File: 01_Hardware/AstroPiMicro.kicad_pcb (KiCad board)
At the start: 2 copper layers, 65 x 50.2 mm, 53 parts, among them J1 RPi Connector, J10 6-pin JST PH, J2 USB_C_Receptacle_USB2.0, J3 2-pin JST PH, J4 4-pin JST SH, J5 4-pin JST SH, J6 11-pin JST PH, J7 3-pin JST PH, J8 3-pin JST PH, J9 6-pin JST PH, SW1 SW-ON-OFF, U1 LM809, U2 STM32G431KBTx, U3 MCP73831-2-OT, U4 TPS61090, U5 Joystick, Y1 16MHz

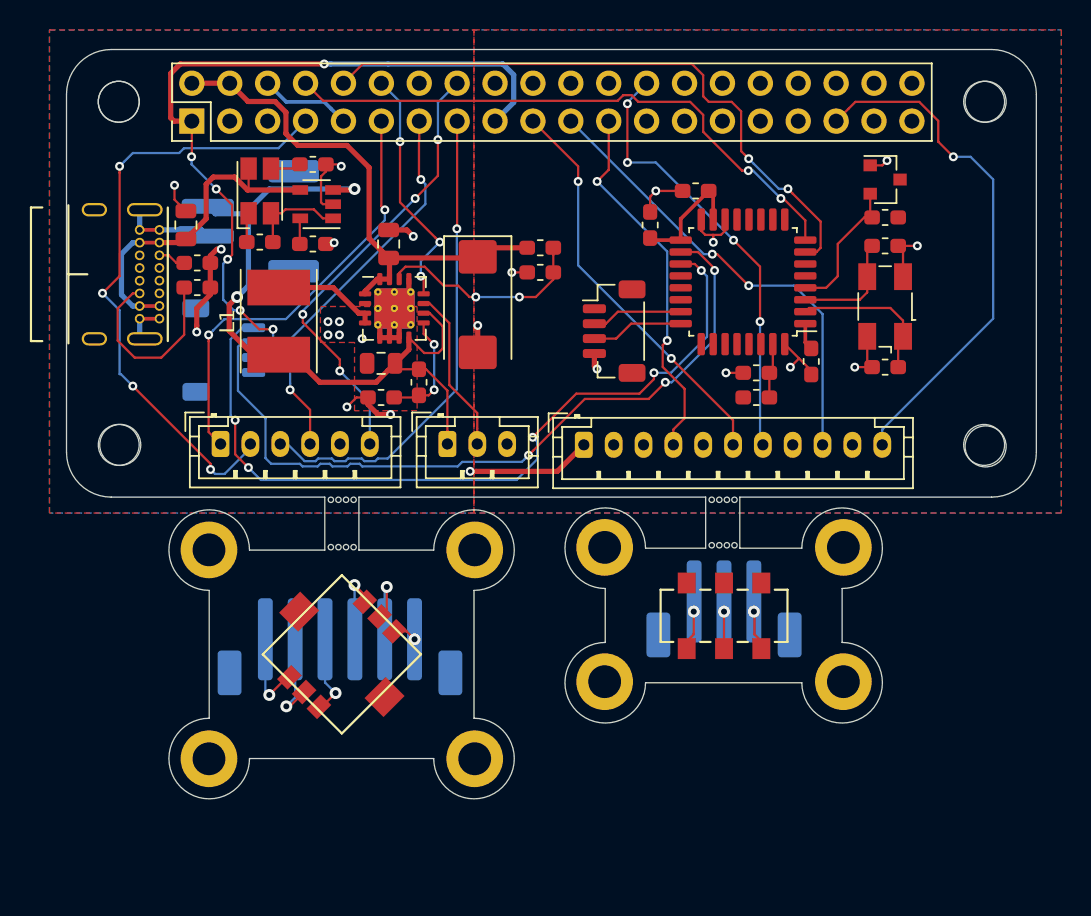
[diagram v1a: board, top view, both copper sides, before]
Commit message: Started on HW version 2
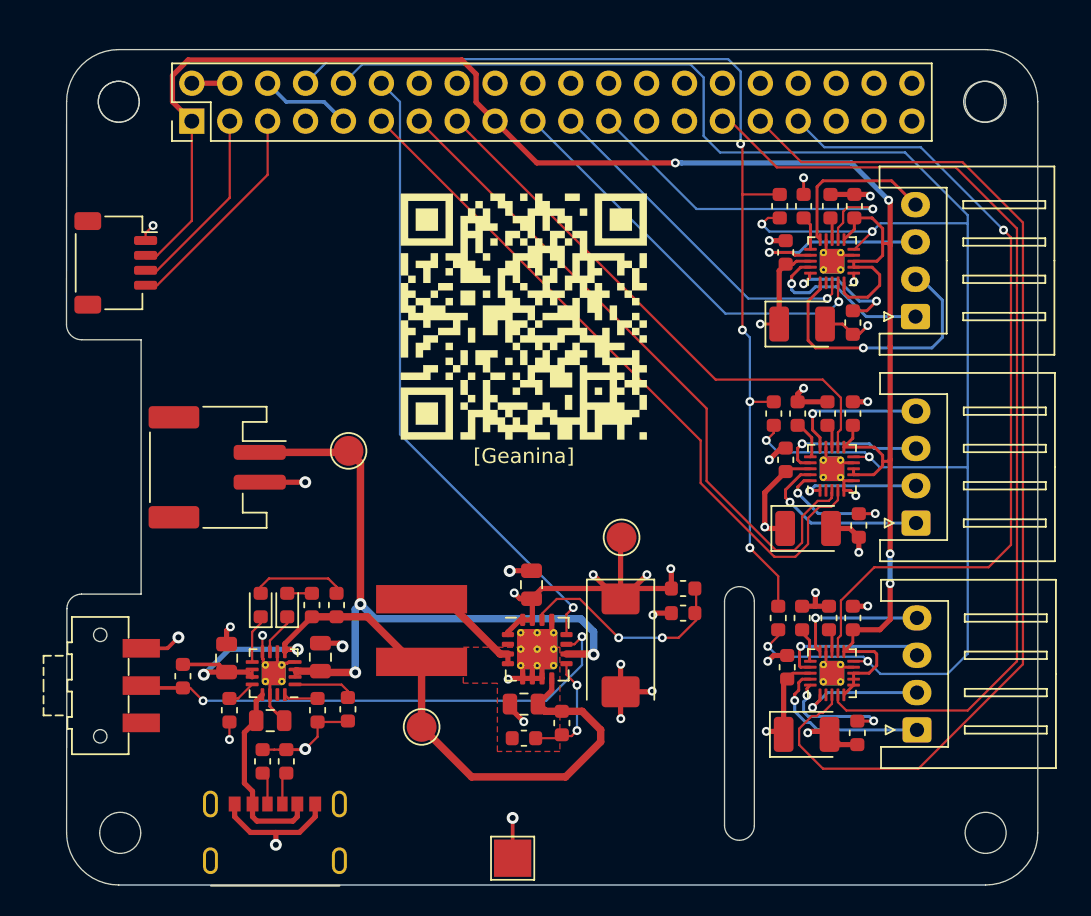
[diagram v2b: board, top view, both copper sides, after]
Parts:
- removed the ? at (53.6, 75.5)
- removed the ? at (111.6, 75.6)
- removed G***: LOGO, astropi:qr
- removed J10: 6-pin JST PH, Connector_JST:JST_PH_B6B-PH-K_1x06_P2.00mm_Vertical
- removed J8: 3-pin JST PH, Connector_JST:JST_PH_B3B-PH-SM4-TB_1x03-1MP_P2.00mm_Vertical
- removed J9: 6-pin JST PH, Connector_JST:JST_PH_B6B-PH-SM4-TB_1x06-1MP_P2.00mm_Vertical
- removed REF** (x8): MountingHole_2.2mm_M2_ISO14580_Pad, MountingHole:MountingHole_2.2mm_M2_ISO14580_Pad
- removed Y1: 16MHz, Crystal:Crystal_SMD_Abracon_ABM3B-4Pin_5.0x3.2mm
- added ?: , RPi_Hat:RPi_Hat_Mounting_Hole, F.Cu at (53.6, 101.5)
- added ?: , RPi_Hat:RPi_Hat_Mounting_Hole, F.Cu at (111.6, 101.5)
- added C11: 100nF, Capacitor_SMD:C_0603_1608Metric, F.Cu at (102.7, 73.4)
- added C12: 100nF, Capacitor_SMD:C_0603_1608Metric, F.Cu at (98.2, 62.6)
- added C13: 47uF, Capacitor_Tantalum_SMD:CP_EIA-3528-15_AVX-H, F.Cu at (99.3, 67.4)
- added C14: 100nF, Capacitor_SMD:C_0603_1608Metric, F.Cu at (101.2, 59.5)
- added C15: 100nF, Capacitor_SMD:C_0603_1608Metric, F.Cu at (102.7, 87.1)
- added C16: 100nF, Capacitor_SMD:C_0603_1608Metric, F.Cu at (98.3, 90.4)
- added C17: 47uF, Capacitor_Tantalum_SMD:CP_EIA-3528-15_AVX-H, F.Cu at (99.6, 94.9)
- added C18: 100nF, Capacitor_SMD:C_0603_1608Metric, F.Cu at (101.1, 87.1)
- added C3: 4.7uF, Capacitor_SMD:C_0805_2012Metric, F.Cu at (67.0, 89.7)
- added D2: Orange, LED_SMD:LED_0603_1608Metric, F.Cu at (63.0, 86.2)
- added QR*****: MiniCalinGeani, astropi:MiniCalinGeani, F.Cu at (80.7, 66.9)
- added R11: 0.75, Resistor_SMD:R_0603_1608Metric, F.Cu at (99.0, 73.4)
- added R14: 0.75, Resistor_SMD:R_0603_1608Metric, F.Cu at (103.1, 80.9)
- added R15: 1k, Resistor_SMD:R_0603_1608Metric, F.Cu at (97.8, 59.5)
- added R16: 220m, Resistor_SMD:R_0603_1608Metric, F.Cu at (99.4, 59.5)
- added R17: 220m, Resistor_SMD:R_0603_1608Metric, F.Cu at (102.7, 67.3)
- added R18: 1k, Resistor_SMD:R_0603_1608Metric, F.Cu at (97.7, 87.1)
- added R19: 220m, Resistor_SMD:R_0603_1608Metric, F.Cu at (99.3, 87.1)
- added R20: 220m, Resistor_SMD:R_0603_1608Metric, F.Cu at (103.0, 94.8)
- added R21: 10k, Resistor_SMD:R_0603_1608Metric, F.Cu at (57.8, 91.0)
- added TP1: TP_VBAT, TestPoint:TestPoint_Pad_D2.0mm, F.Cu at (68.9, 75.9)
- added TP2: TP_Supply, TestPoint:TestPoint_Pad_D2.0mm, F.Cu at (73.8, 94.4)
- added TP3: TP_5V, TestPoint:TestPoint_Pad_D2.0mm, F.Cu at (87.2, 81.7)
- added TP4: TP_GND, TestPoint:TestPoint_Pad_2.5x2.5mm, F.Cu at (79.9, 103.2)
- C1: value 27pF -> 100nF; footprint Capacitor_SMD:C_0603_1608Metric_Pad1.05x0.95mm_HandSolder -> Capacitor_SMD:C_0603_1608Metric
- C10: footprint Capacitor_Tantalum_SMD:CP_EIA-7343-31_Kemet-D_Pad2.25x2.55mm_HandSolder -> Capacitor_Tantalum_SMD:CP_EIA-7343-15_Kemet-W
- C2: value 27pF -> 1uF; footprint Capacitor_SMD:C_0603_1608Metric_Pad1.05x0.95mm_HandSolder -> Capacitor_SMD:C_0805_2012Metric
- C4: value 100nF -> 10uF; footprint Capacitor_SMD:C_0603_1608Metric_Pad1.05x0.95mm_HandSolder -> Capacitor_SMD:C_0805_2012Metric
- C5: value 10uF -> 100nF; footprint Capacitor_SMD:C_0805_2012Metric -> Capacitor_SMD:C_0603_1608Metric
- C6: value 100nF -> 47uF; footprint Capacitor_SMD:C_0603_1608Metric_Pad1.05x0.95mm_HandSolder -> Capacitor_Tantalum_SMD:CP_EIA-3528-15_AVX-H
- C7: footprint Capacitor_SMD:C_0603_1608Metric_Pad1.05x0.95mm_HandSolder -> Capacitor_SMD:C_0603_1608Metric
- D1: value Status LED -> Green; footprint LED_SMD:LED_Avago_PLCC4_3.2x2.8mm_CW -> LED_SMD:LED_0603_1608Metric
- J2: value USB_C_Receptacle_USB2.0 -> SHOU_HAN_TYPE-C_6P; footprint astropi:USB_C_GCT_USB4085 -> astropi:SHOU HAN TYPE-C 6P
- J3, J4: moved to F.Cu
- J5: value 4-pin JST SH -> Stepper_Focus; footprint Connector_JST:JST_SH_BM04B-SRSS-TB_1x04-1MP_P1.00mm_Vertical -> Connector_JST:JST_XH_S4B-XH-A_1x04_P2.50mm_Horizontal
- J6: value 11-pin JST PH -> Stepper_Azimuth; footprint Connector_JST:JST_PH_B11B-PH-K_1x11_P2.00mm_Vertical -> Connector_JST:JST_XH_S4B-XH-A_1x04_P2.50mm_Horizontal
- J7: value 3-pin JST PH -> Stepper_Altitude; footprint Connector_JST:JST_PH_B3B-PH-K_1x03_P2.00mm_Vertical -> Connector_JST:JST_XH_S4B-XH-A_1x04_P2.50mm_Horizontal
- L1: value 6.8uH -> 10uH; footprint Inductor_SMD:L_Taiyo-Yuden_NR-50xx_HandSoldering -> astropi:VLS6045EX-100M
- R1: value 10k -> 1.1k; footprint Resistor_SMD:R_0603_1608Metric_Pad1.05x0.95mm_HandSolder -> Resistor_SMD:R_0603_1608Metric
- R10, R12, R13, R4, R5, R7, R8, R9: footprint Resistor_SMD:R_0603_1608Metric_Pad1.05x0.95mm_HandSolder -> Resistor_SMD:R_0603_1608Metric
- R2: value 10k -> 1k; footprint Resistor_SMD:R_0603_1608Metric_Pad1.05x0.95mm_HandSolder -> Resistor_SMD:R_0603_1608Metric
- R3: value 10k -> 1.5k; footprint Resistor_SMD:R_0603_1608Metric_Pad1.05x0.95mm_HandSolder -> Resistor_SMD:R_0603_1608Metric
- R6: value 2k -> 10k; footprint Resistor_SMD:R_0603_1608Metric_Pad1.05x0.95mm_HandSolder -> Resistor_SMD:R_0603_1608Metric
- SW1: value SW-ON-OFF -> SW_SPDT; footprint astropi:SSSS213202 -> Button_Switch_SMD:SW_SPDT_CK-JS102011SAQN
- U1: value LM809 -> BQ24074RGT; footprint Package_TO_SOT_SMD:SOT-23 -> Package_DFN_QFN:VQFN-16-1EP_3x3mm_P0.5mm_EP1.6x1.6mm_ThermalVias
- U2: value STM32G431KBTx -> TMC2300; footprint Package_QFP:LQFP-32_7x7mm_P0.8mm -> Package_DFN_QFN:QFN-20-1EP_3x3mm_P0.4mm_EP1.65x1.65mm_ThermalVias
- U3: value MCP73831-2-OT -> TMC2300; footprint Package_TO_SOT_SMD:SOT-23-5 -> Package_DFN_QFN:QFN-20-1EP_3x3mm_P0.4mm_EP1.65x1.65mm_ThermalVias
- U5: value Joystick -> TMC2300; footprint astropi:SKRHAAE010 -> Package_DFN_QFN:QFN-20-1EP_3x3mm_P0.4mm_EP1.65x1.65mm_ThermalVias
- moved R1 55.0 mm to (60.9, 93.3), turned to 90 degrees
- moved U1 52.7 mm to (63.9, 90.8), turned to 180 degrees
- moved C2 52.1 mm to (63.6, 94.0)
- moved C4 43.9 mm to (60.7, 89.8), turned to 90 degrees
- moved C5 43.2 mm to (98.2, 76.5)
- moved SW1 39.4 mm to (52.3, 91.6), turned to 270 degrees
- moved J2 38.1 mm to (64.0, 99.6), turned to 0 degrees
- moved J7 36.8 mm to (107.0, 94.6), turned to 90 degrees
- moved R3 36.1 mm to (66.8, 93.3), turned to 90 degrees
- moved U3 34.8 mm to (101.3, 63.2), turned to 90 degrees
- moved R4 33.7 mm to (63.1, 96.7), turned to 270 degrees
- moved U5 32.9 mm to (101.3, 90.8), turned to 90 degrees
- moved R5 32.3 mm to (64.7, 96.7), turned to 270 degrees
- moved R6 31.3 mm to (68.9, 93.2), turned to 270 degrees
- moved R8 29.6 mm to (68.1, 86.2), turned to 90 degrees
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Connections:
- C1 pad 1: Net-(C1-Pad1) -> +3V3
- C2 pad 1: Net-(C2-Pad1) -> VBUS
- C4 pad 1: +3V3 -> /Vsupply
- C5 pad 1: VBUS -> +5V
- C6 pad 1: +3V3 -> +5V
- C7 pad 1: +3V3 -> Net-(C7-Pad1)
- C8 pad 1: +BATT -> /Vsupply
- D1 pad 2: VBUS -> Net-(D1-Pad2)
- J1 pad 10: /PI_UART_RX -> /UART_RX
- J1 pad 11: /GPIO17 -> /STEP_Focus
- J1 pad 13: /GPIO27 -> /DIR_Focus
- J1 pad 15: /GPIO22 -> /ERR_Focus
- J1 pad 16: /GPIO23 -> (no net)
- J1 pad 18: Net-(J1-Pad18) -> (no net)
- J1 pad 19: /LCD_MOSI -> /STEP_Az
- J1 pad 21: /LCD_TDC -> /DIR_Az
- J1 pad 22: Net-(J1-Pad22) -> (no net)
- J1 pad 23: /LCD_SCK -> /ERR_Az
- J1 pad 24: Net-(J1-Pad24) -> (no net)
- J1 pad 26: /LCD_~TCS -> (no net)
- J1 pad 27: Net-(J1-Pad27) -> (no net)
- J1 pad 28: Net-(J1-Pad28) -> (no net)
- J1 pad 29: Net-(J1-Pad29) -> /STEP_Alt
- J1 pad 3: Net-(J1-Pad3) -> /IMU_SDA
- J1 pad 31: Net-(J1-Pad31) -> /DIR_Alt
- J1 pad 32: Net-(J1-Pad32) -> (no net)
- J1 pad 33: Net-(J1-Pad33) -> /ERR_Alt
- J1 pad 35: /LCD_BL -> (no net)
- J1 pad 36: Net-(J1-Pad36) -> (no net)
- J1 pad 37: Net-(J1-Pad37) -> (no net)
- J1 pad 38: Net-(J1-Pad38) -> (no net)
- J1 pad 40: Net-(J1-Pad40) -> (no net)
- J1 pad 5: Net-(J1-Pad5) -> /IMU_SCL
- J1 pad 7: /GPIO4 -> (no net)
- J1 pad 8: /PI_UART_TX -> /UART_TX
- J5 pad 1: +3V3 -> /Focus_A1
- J5 pad 2: /SWDIO -> /Focus_A2
- J5 pad 3: /SWCLK -> /Focus_B1
- J5 pad 4: GND -> /Focus_B2
- J6 pad 1: +5V -> /Az_A1
- J6 pad 2: /LCD_3V3 -> /Az_A2
- J6 pad 3: GND -> /Az_B1
- J6 pad 4: /LCD_SCK -> /Az_B2
- J7 pad 1: +BATT -> /Alt_A1
- J7 pad 2: /ON\~OFF -> /Alt_A2
- J7 pad 3: GND -> /Alt_B1
- L1 pad 1: +BATT -> /Vsupply
- R1 pad 1: +3V3 -> GND
- R1 pad 2: /~RESET -> Net-(R1-Pad2)
- R2 pad 1: Net-(R2-Pad1) -> /UART_TX
- R2 pad 2: GND -> /UART_RX
- R3 pad 1: +3V3 -> GND
- R3 pad 2: Net-(R2-Pad1) -> Net-(R3-Pad2)
- R7 pad 1: Net-(D1-Pad1) -> /Vsupply
- R7 pad 2: /CHG_ST -> Net-(D1-Pad2)
- R8 pad 1: Net-(D1-Pad3) -> /Vsupply
- R8 pad 2: GND -> Net-(D2-Pad2)
- R9 pad 1: +BATT -> /Vsupply
- SW1 pad 1: /SW_1 -> GND
- SW1 pad 2: /SW_2 -> /ON\~OFF
- SW1 pad 3: /SW_3 -> (no net)
- U1 pad 1: GND -> Net-(R6-Pad1)
- U1 pad 2: /~RESET -> +BATT
- U1 pad 3: +3V3 -> +BATT
- U2 pad 1: +3V3 -> /Focus_A2
- U2 pad 10: Net-(U2-Pad10) -> /UART_RX
- U2 pad 11: Net-(U2-Pad11) -> +3V3
- U2 pad 12: Net-(U2-Pad12) -> /ERR_Focus
- U2 pad 13: Net-(U2-Pad13) -> Net-(C7-Pad1)
- U2 pad 15: +3V3 -> /Focus_B2
- U2 pad 16: GND -> Net-(R11-Pad1)
- U2 pad 17: +3V3 -> /Focus_B1
- U2 pad 18: /IMU_SDA -> +5V
- U2 pad 19: /IMU_SCL -> /Focus_A1
- U2 pad 2: Net-(C1-Pad1) -> (no net)
- U2 pad 21: Net-(U2-Pad21) -> GND
- U2 pad 3: Net-(C2-Pad1) -> /DIR_Focus
- U2 pad 4: /~RESET -> /STEP_Focus
- U2 pad 5: Net-(U2-Pad5) -> GND
- U2 pad 6: Net-(U2-Pad6) -> GND
- U2 pad 7: /PI_UART_RX -> +3V3
- U2 pad 8: /PI_UART_TX -> +3V3
- U2 pad 9: Net-(U2-Pad9) -> GND
- U3 pad 1: /CHG_ST -> /Az_A2
- U3 pad 2: GND -> (no net)
- U3 pad 3: +BATT -> /DIR_Az
- U3 pad 4: VBUS -> /STEP_Az
- U3 pad 5: Net-(R6-Pad1) -> +3V3
- U4 pad 2: Net-(U4-Pad2) -> (no net)
- U4 pad 8: +BATT -> /Vsupply
- U5 pad 1: /JOY_A -> /Alt_A2
- U5 pad 2: /JOY_PUSH -> (no net)
- U5 pad 3: /JOY_C -> /DIR_Alt
- U5 pad 4: /JOY_B -> /STEP_Alt
- U5 pad 5: /JOY_GND -> +3V3
- U5 pad 6: /JOY_D -> +3V3
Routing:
- net /UART_RX: track 0.00 -> 129.2 mm, vias 0 -> 6
- net /DIR_Alt: track 0.00 -> 73.1 mm
- net /UART_TX: track 0.00 -> 71.2 mm, vias 0 -> 4
- net +3V3: track 62.1 -> 130.2 mm, vias 6 -> 4
- net /STEP_Alt: track 0.00 -> 65.8 mm
- net /ERR_Alt: track 0.00 -> 54.5 mm, vias 0 -> 1
- net /Vsupply: track 0.00 -> 53.3 mm, vias 0 -> 2
- net /STEP_Focus: track 0.00 -> 47.6 mm
- net /DIR_Focus: track 0.00 -> 45.4 mm
- net /PI_UART_RX: track 42.2 -> 0.00 mm, vias 2 -> 0
- net /GPIO4: track 41.3 -> 0.00 mm, vias 4 -> 0
- net /PI_UART_TX: track 39.6 -> 0.00 mm, vias 2 -> 0
- net /IMU_SCL: track 53.7 -> 14.8 mm, vias 5 -> 0
- net /IMU_SDA: track 51.0 -> 12.8 mm, vias 3 -> 0
- net /ERR_Focus: track 0.00 -> 36.8 mm
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- added copper zone on In1, net +5V
- added copper zone on In2, net GND
- removed copper zone on F.Cu, net +3V3
- removed copper zone on F.Cu, net +5V
- removed copper zone on B.Cu, net GND
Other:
- board size 65 x 50.2 mm -> 65.1 x 56 mm
- copper layers 2 -> 4
- board text removed: "<NP"
